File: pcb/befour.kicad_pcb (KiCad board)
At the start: 2 copper layers, 160 x 100 mm, 114 parts, among them J1 USB_C_Receptacle_PowerOnly_6P, J2 READOUT, J3 DEVICES, J5 Conn_01x40_Pin, SW1 SW_SPDT, SW2 PRG_SELECT, SW3 SW_Push, SW4 SW_Push, SW5 SW_SPDT, U1 74LS14, U10 74LS11, U11 ALU_ADD, U12 ALU_NAND, U13 SI_BUFFER, U14 74LS00, U15 CLKDIV, U16 74LS14, U17 MISC, U18 ALU_NAND_BUFFER, U19 74LS11, U2 MEMORY, U20 74LS11, U21 A_BUFFER, U22 ALU_ADD_BUFFER, U23 CLKDIV2, U24 AREG, U25 74LS00, U26 XOR_EQUAL, U27 TEMP, U28 BREG, U29 FLAGS_BUFFER, U3 B_OUT_BUFFER, U30 DEVICES_BUFFER, U31 PCH_BUFFER, U32 74LS138, U33 PCL_BUFFER, U34 PCH, U35 PCL, U36 ADR_BUFFER, U37 SI_ADR_BUFFER, U4 DB_OUT_BUFFER, U5 INSTSTORe, U6 TEMP_BUFFER, U7 B_BUFFER, U8 74LS125, U9 74LS138, X1 1MHz

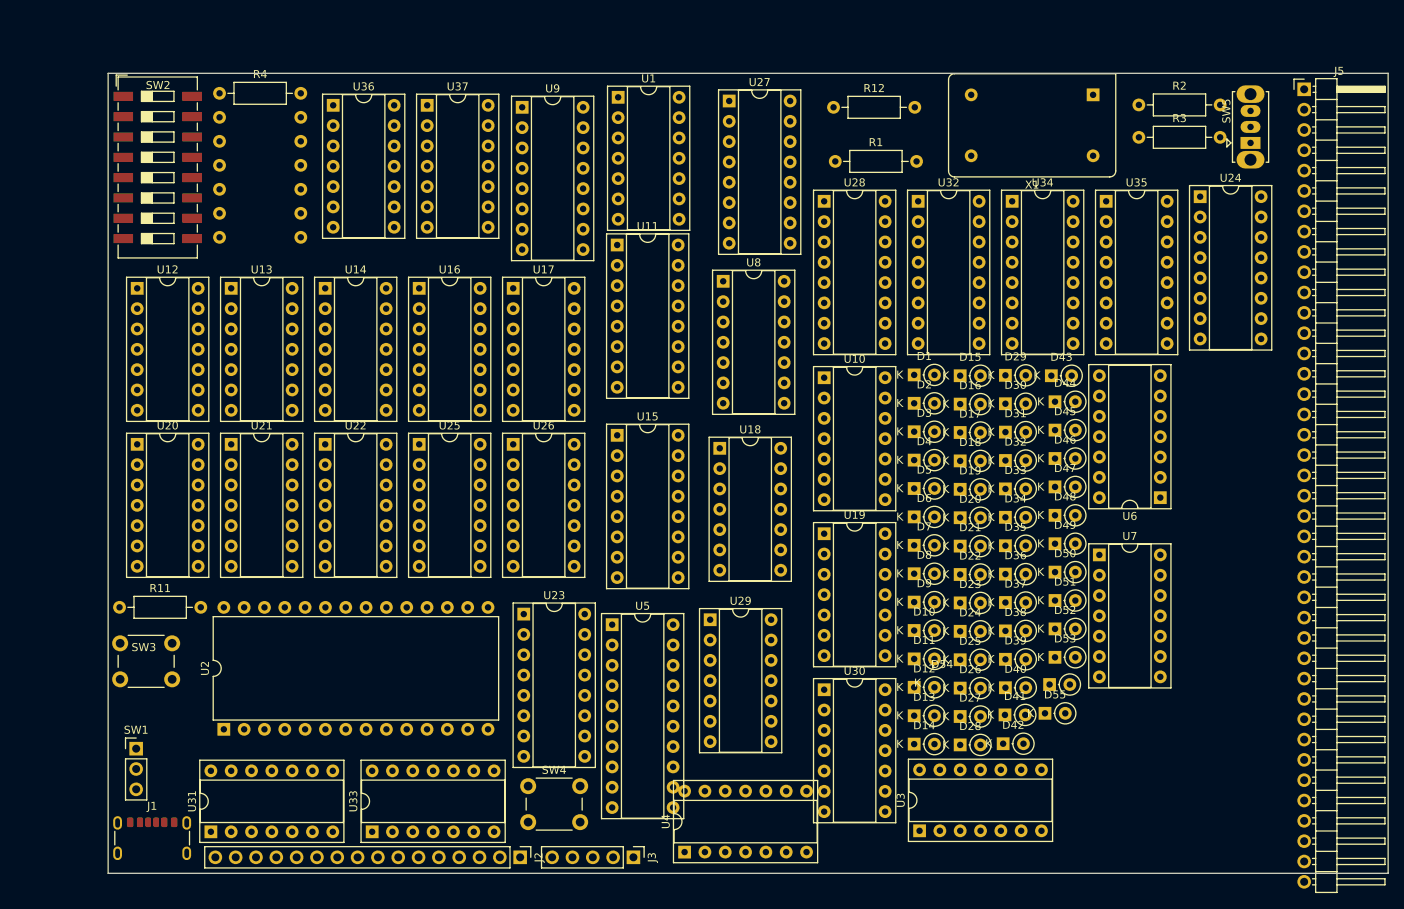
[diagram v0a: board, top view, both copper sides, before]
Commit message: PCB
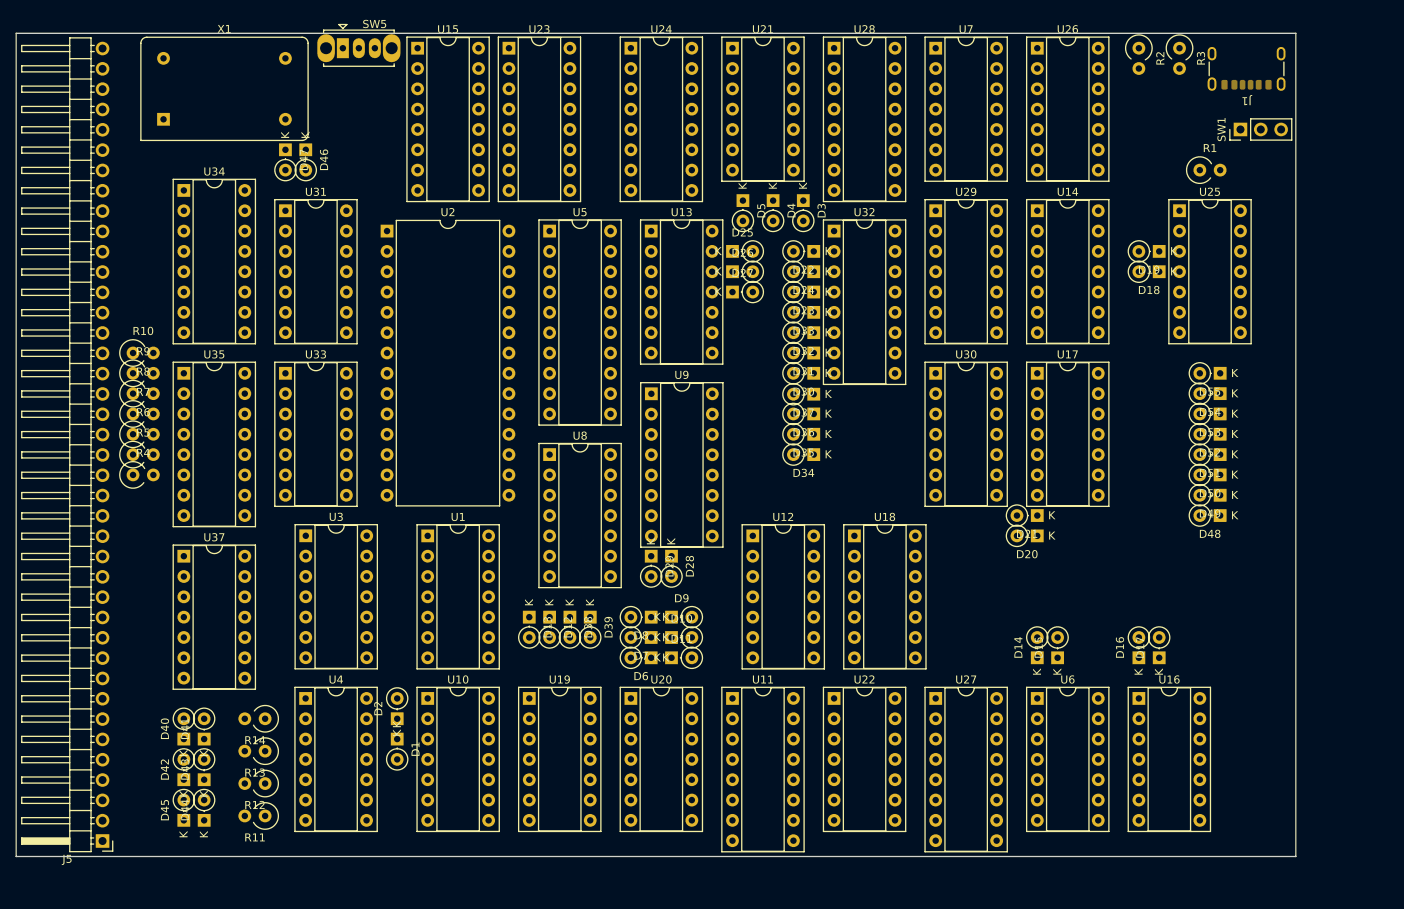
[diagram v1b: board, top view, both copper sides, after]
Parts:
- removed J2: READOUT, Connector_PinHeader_2.54mm:PinHeader_1x16_P2.54mm_Vertical
- removed J3: DEVICES, Connector_PinHeader_2.54mm:PinHeader_1x05_P2.54mm_Vertical
- removed SW2: PRG_SELECT, Button_Switch_SMD:SW_DIP_SPSTx08_Slide_9.78x22.5mm_W8.61mm_P2.54mm
- removed SW3, SW4: SW_Push, Button_Switch_THT:SW_PUSH_6mm_H5mm
- removed U36: ADR_BUFFER, Package_DIP:DIP-14_W7.62mm_Socket
- added R13: 10K, Resistor_THT:R_Axial_DIN0309_L9.0mm_D3.2mm_P2.54mm_Vertical, F.Cu at (71.1, 110.7)
- added R14: 10K, Resistor_THT:R_Axial_DIN0309_L9.0mm_D3.2mm_P2.54mm_Vertical, F.Cu at (71.1, 106.7)
- R1, R2, R3, R4: footprint Resistor_THT:R_Axial_DIN0207_L6.3mm_D2.5mm_P10.16mm_Horizontal -> Resistor_THT:R_Axial_DIN0309_L9.0mm_D3.2mm_P2.54mm_Vertical
- R10, R5, R6, R7, R8, R9: footprint Resistor_THT:R_Axial_DIN0207_L6.3mm_D2.5mm_P10.16mm_Horizontal -> Resistor_THT:R_Axial_DIN0309_L9.0mm_D3.2mm_P2.54mm_Vertical; moved to F.Cu
- R11, R12: value 10k -> 10K; footprint Resistor_THT:R_Axial_DIN0207_L6.3mm_D2.5mm_P10.16mm_Horizontal -> Resistor_THT:R_Axial_DIN0309_L9.0mm_D3.2mm_P2.54mm_Vertical
- moved J5 177.2 mm to (50.8, 122.0), turned to 180 degrees
- moved J1 168.5 mm to (193.8, 24.3), turned to 180 degrees
- moved SW1 158.3 mm to (193.0, 33.0), turned to 90 degrees
- moved D45 119.3 mm to (61.0, 119.4), turned to 90 degrees
- moved D44 118.5 mm to (63.5, 119.4), turned to 90 degrees
- moved D43 117.3 mm to (63.5, 114.3), turned to 90 degrees
- moved U35 117.3 mm to (61.0, 63.5)
- moved X1 116.2 mm to (58.4, 31.8), turned to 0 degrees
- moved SW5 114.1 mm to (80.8, 22.9), turned to 0 degrees
- moved R12 110.4 mm to (71.1, 114.8), turned to 180 degrees
- moved D47 105.0 mm to (73.7, 35.6), turned to -90 degrees
- moved U34 103.5 mm to (61.0, 40.6)
- moved U16 103.5 mm to (180.3, 104.1)
- moved D40 102.9 mm to (61.0, 109.2), turned to 90 degrees
- moved D42 102.5 mm to (61.0, 114.3), turned to 90 degrees
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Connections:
- net MANUALCLK renamed EXTCLK
- J5 pad 29: DATAENTRY -> unconnected-(J5-Pin_29-Pad29)
- R11 pad 1: RESET -> +5V
- R11 pad 2: +5V -> /A7
- R12 pad 1: Net-(SW5-A) -> +5V
- R12 pad 2: +5V -> /A6
- U17 pad 1: Net-(U16-Pad4) -> ADD
- U17 pad 2: Net-(U12-Pad3) -> COUT
- U17 pad 3: /ALU0 -> Net-(D20-A)
- U18 pad 1: ADD -> Net-(U16-Pad4)
- U18 pad 2: COUT -> Net-(U12-Pad3)
- U18 pad 3: Net-(D20-A) -> /ALU0
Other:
- board size 160 x 100 mm -> 160 x 102.9 mm
